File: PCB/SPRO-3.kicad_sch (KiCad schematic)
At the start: 53 parts, among them J1 Screw_Terminal_01x02, J2 Micro_SD_Card, J3 Conn_01x22, J4 Conn_01x22, Q1 IRF4905, U1 TSR_1-2450, U2 ESP32-S3-DEVKITC-1-N8R2, U6 LD1117V33

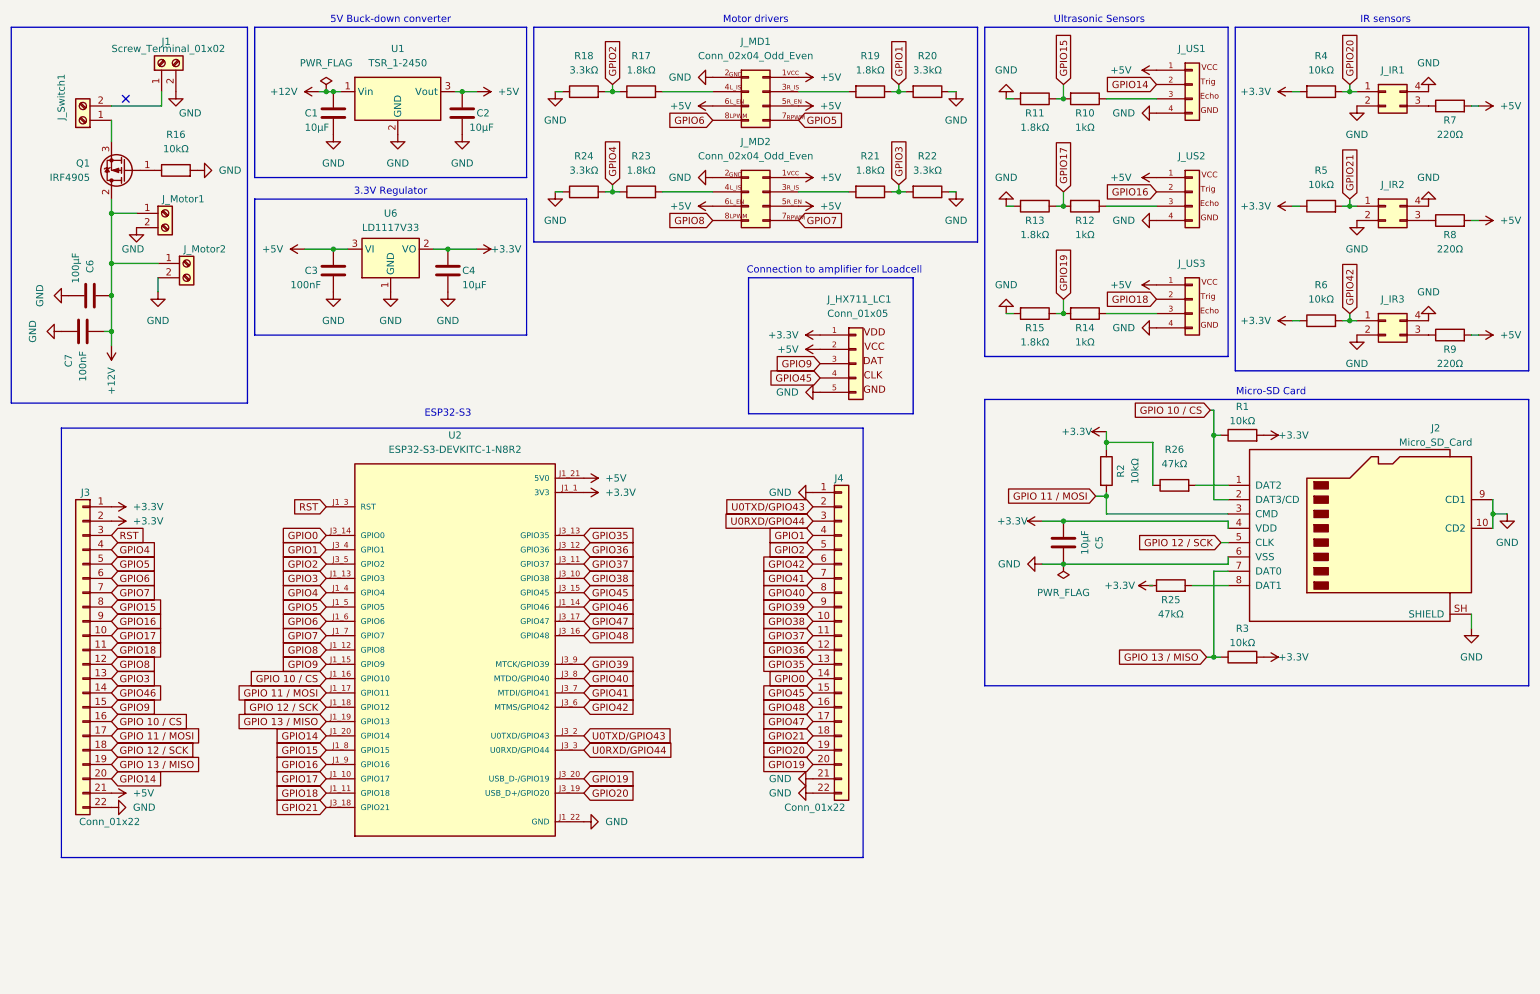
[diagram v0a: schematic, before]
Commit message: Add files via upload
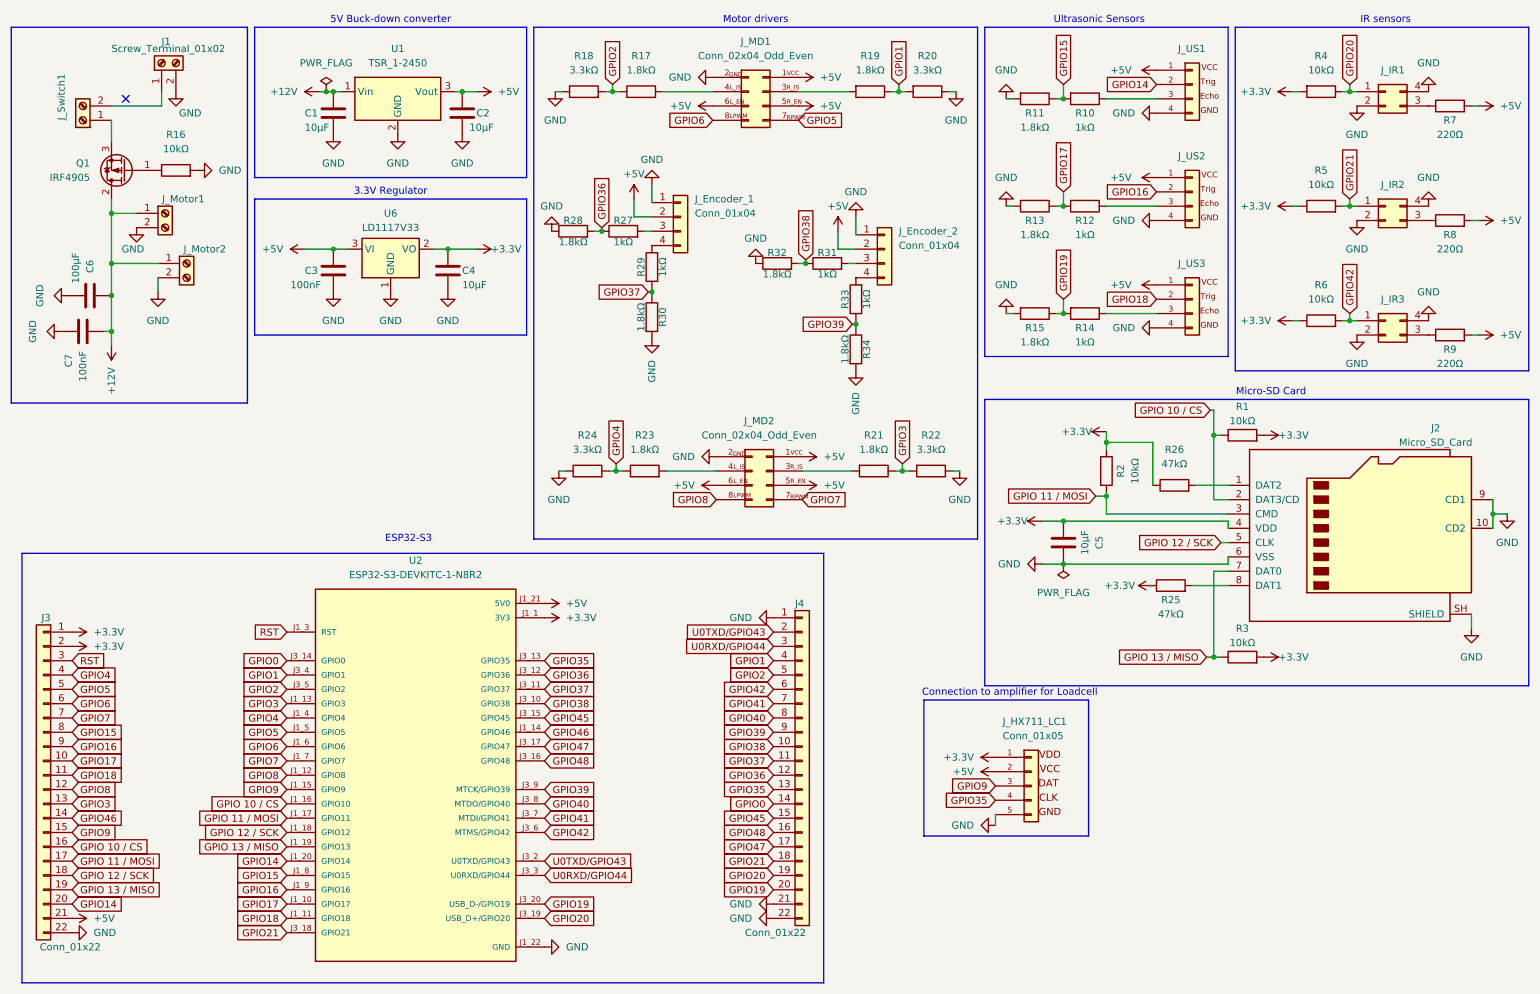
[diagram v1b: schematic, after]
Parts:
- added J_Encoder_1, J_Encoder_2: Conn_01x04, Connector_PinHeader_2.54mm:PinHeader_1x04_P2.54mm_Vertical, symbol Connector_Generic:Conn_01x04
- added R27, R29, R31, R33: 1kΩ, Resistor_THT:R_Axial_DIN0207_L6.3mm_D2.5mm_P7.62mm_Horizontal, symbol Device:R
- added R28, R30, R32, R34: 1.8kΩ, Resistor_THT:R_Axial_DIN0207_L6.3mm_D2.5mm_P7.62mm_Horizontal, symbol Device:R
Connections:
- net +5V: now also J_Encoder_1.2 (Pin_2), J_Encoder_2.2 (Pin_2)
- net GND: now also J_Encoder_1.1 (Pin_1), J_Encoder_2.1 (Pin_1), R28.1, R30.2, R32.1, R34.2
- net GPIO35: now also J_HX711_LC1.4 (Pin_4)
- net GPIO36: now also R27.1, R28.2
- net GPIO37: now also R29.1, R30.1
- net GPIO38: now also R31.1, R32.2
- net GPIO39: now also R33.1, R34.1
- net GPIO45: no longer J_HX711_LC1.4 (Pin_4)
- new net: J_Encoder_1.3 (Pin_3), R27.2
- new net: J_Encoder_2.4 (Pin_4), R33.2
- new net: J_Encoder_2.3 (Pin_3), R31.2
- new net: J_Encoder_1.4 (Pin_4), R29.2
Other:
- moved on the sheet: J3, J4, J_HX711_LC1, J_MD2, R21, R22, R23, R24, U2
